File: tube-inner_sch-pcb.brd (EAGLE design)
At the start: 4 x 70 mm, 13 parts

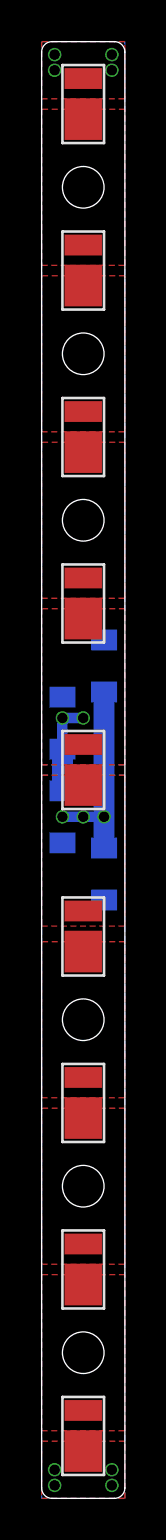
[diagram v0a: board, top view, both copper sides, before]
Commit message: Progress
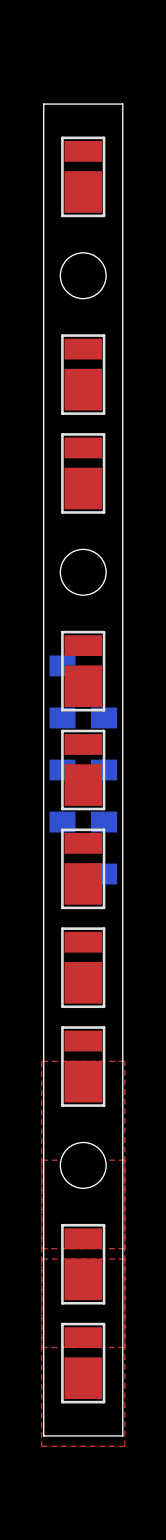
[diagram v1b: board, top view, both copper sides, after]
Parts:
- added D14: 3500K, OPTO:JE2835AWT
- moved D8 9.75 mm to (0.00, -14.2)
- moved D9 8.25 mm to (0.00, -23.8)
- moved D7 6.50 mm to (0.00, -9.50)
- moved D2 5.00 mm to (0.00, 19.0)
- moved D13 3.75 mm to (1.00, 1.25)
- moved D1 3.50 mm to (0.00, 28.5)
- moved D4 3.25 mm to (0.00, 4.75)
- moved D6 3.25 mm to (0.00, -4.75)
- moved D3 1.75 mm to (0.00, 14.2)
- moved D11 1.50 mm to (-1.00, 3.75)
- moved D12 1.25 mm to (1.00, -3.75)
- moved D10 1.00 mm to (-1.00, -1.25)
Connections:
- new net N$7: D14.A, D9.K
- net CATHODE: now also D14.K; no longer D9.K
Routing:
- net CATHODE: track 11.0 -> 0.00 mm, vias 7 -> 0
- net ANODE: track 4.50 -> 0.00 mm, vias 6 -> 0
- removed copper zone on layer 1, net ANODE
- removed copper zone on layer 2, net ANODE
- removed copper zone on layer 1, net CATHODE
- removed copper zone on layer 2, net CATHODE
- removed copper zone on layer 16, net IN1
- removed copper zone on layer 16, net IN2
- removed copper zone on layer 1, net N$1
- removed copper zone on layer 1, net N$19
- removed copper zone on layer 1, net N$2
- removed copper zone on layer 1, net N$3
- removed copper zone on layer 1, net N$4
- removed copper zone on layer 1, net N$5
- removed copper zone on layer 1, net N$6
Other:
- board size 4 x 70 mm -> 3.8 x 64 mm
